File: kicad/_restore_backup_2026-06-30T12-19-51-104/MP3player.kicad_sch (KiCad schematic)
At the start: 0 parts

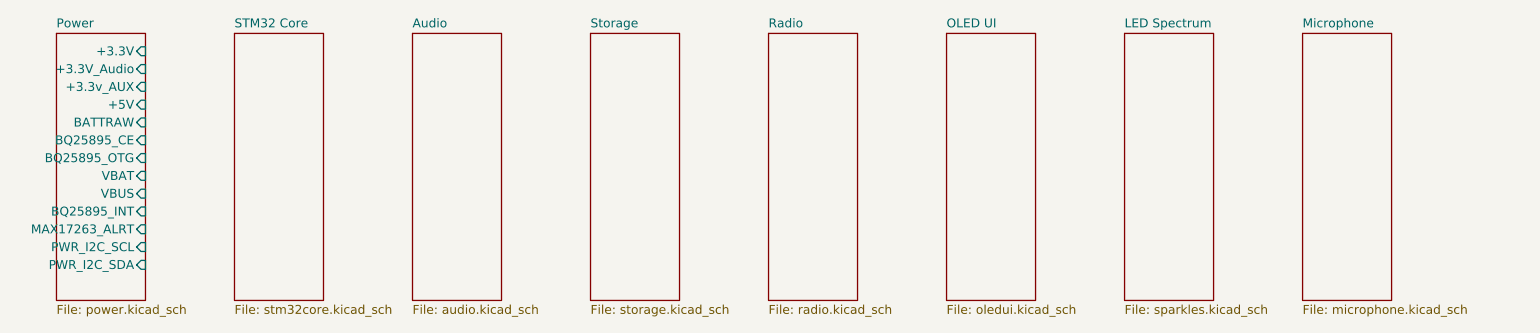
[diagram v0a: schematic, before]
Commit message: updates
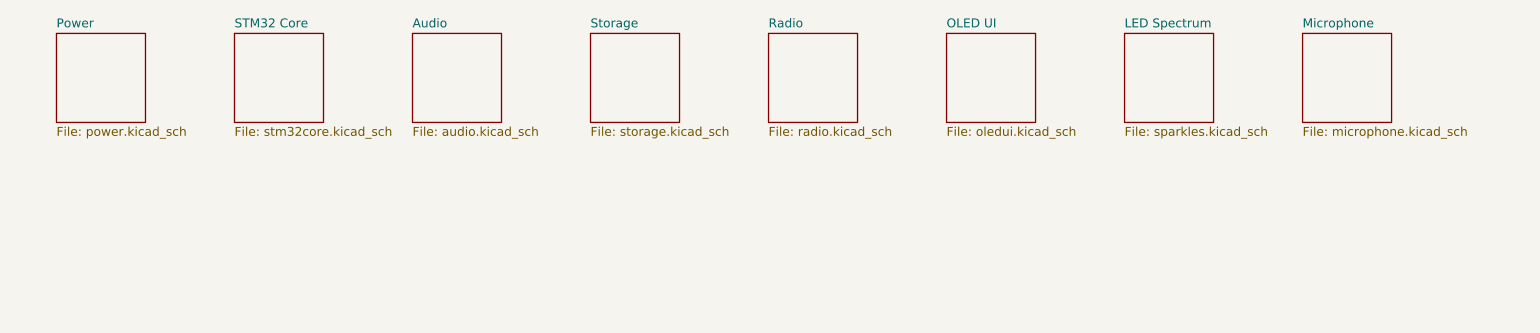
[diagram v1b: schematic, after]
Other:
- sheet Power ports: added none; removed +3.3V, +3.3V_Audio, +3.3v_AUX, +5V, BATTRAW, BQ25895_CE, BQ25895_INT, BQ25895_OTG, MAX17263_ALRT, PWR_I2C_SCL, PWR_I2C_SDA, VBAT, VBUS
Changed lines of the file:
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@@
 	(sheet
 		(at 203.2 25.4)
-		(size 12.7 38.1)
+		(size 12.7 12.7)
 		(exclude_from_sim no)
 		(in_bom yes)
@@
 		)
 		(property "Sheetfile" "microphone.kicad_sch"
-			(at 203.2 64.0846 0)
+			(at 203.2 38.6846 0)
 			(show_name no)
 			(do_not_autoplace no)
@@
 	(sheet
 		(at 25.4 25.4)
-		(size 12.7 38.1)
+		(size 12.7 12.7)
 		(exclude_from_sim no)
 		(in_bom yes)
@@
 		)
 		(property "Sheetfile" "power.kicad_sch"
-			(at 25.4 64.0846 0)
-			(show_name no)
-			(do_not_autoplace no)
-			(effects
-				(font
-					(size 1.27 1.27)
-				)
-				(justify left top)
-			)
-		)
-		(pin "+3.3V" input
-			(at 38.1 27.94 0)
-			(effects
-				(font
-					(size 1.27 1.27)
-				)
-				(justify right)
-			)
-		)
-		(pin "+3.3V_Audio" input
-			(at 38.1 30.48 0)
-			(effects
-				(font
-					(size 1.27 1.27)
-				)
-				(justify right)
-			)
-		)
-		(pin "+5V" input
-			(at 38.1 35.56 0)
-			(effects
-				(font
-					(size 1.27 1.27)
-				)
-				(justify right)
-			)
-		)
-		(pin "BATTRAW" input
-			(at 38.1 38.1 0)
-			(effects
-				(font
-					(size 1.27 1.27)
-				)
-				(justify right)
-			)
-		)
-		(pin "VBAT" input
-			(at 38.1 45.72 0)
-			(effects
-				(font
-					(size 1.27 1.27)
-				)
-				(justify right)
-			)
-		)
-		(pin "VBUS" input
-			(at 38.1 48.26 0)
-			(effects
-				(font
-					(size 1.27 1.27)
-				)
-				(justify right)
-			)
-		)
-		(pin "BQ25895_INT" input
-			(at 38.1 50.8 0)
-			(effects
-				(font
-					(size 1.27 1.27)
-				)
-				(justify right)
-			)
-		)
-		(pin "MAX17263_ALRT" input
-			(at 38.1 53.34 0)
-			(effects
-				(font
-					(size 1.27 1.27)
-				)
-				(justify right)
-			)
-		)
-		(pin "PWR_I2C_SCL" input
-			(at 38.1 55.88 0)
-			(effects
-				(font
-					(size 1.27 1.27)
-				)
-				(justify right)
-			)
-		)
-		(pin "PWR_I2C_SDA" input
-			(at 38.1 58.42 0)
-			(effects
-				(font
-					(size 1.27 1.27)
-				)
-				(justify right)
-			)
-		)
-		(pin "BQ25895_CE" input
-			(at 38.1 40.64 0)
-			(effects
-				(font
-					(size 1.27 1.27)
-				)
-				(justify right)
-			)
-		)
-		(pin "BQ25895_OTG" input
-			(at 38.1 43.18 0)
-			(effects
-				(font
-					(size 1.27 1.27)
-				)
-				(justify right)
-			)
-		)
-		(pin "+3.3v_AUX" input
-			(at 38.1 33.02 0)
-			(effects
-				(font
-					(size 1.27 1.27)
-				)
-				(justify right)
+			(at 25.4 38.6846 0)
+			(show_name no)
+			(do_not_autoplace no)
+			(effects
+				(font
+					(size 1.27 1.27)
+				)
+				(justify left top)
 			)
 		)
@@
 	(sheet
 		(at 152.4 25.4)
-		(size 12.7 38.1)
+		(size 12.7 12.7)
 		(exclude_from_sim no)
 		(in_bom yes)
@@
 		)
 		(property "Sheetfile" "oledui.kicad_sch"
-			(at 152.4 64.0846 0)
+			(at 152.4 38.6846 0)
 			(show_name no)
 			(do_not_autoplace no)
@@
 	(sheet
 		(at 127 25.4)
-		(size 12.7 38.1)
+		(size 12.7 12.7)
 		(exclude_from_sim no)
 		(in_bom yes)
@@
 		)
 		(property "Sheetfile" "radio.kicad_sch"
-			(at 127 64.0846 0)
+			(at 127 38.6846 0)
 			(show_name no)
 			(do_not_autoplace no)
@@
 	(sheet
 		(at 50.8 25.4)
-		(size 12.7 38.1)
+		(size 12.7 12.7)
 		(exclude_from_sim no)
 		(in_bom yes)
@@
 		)
 		(property "Sheetfile" "stm32core.kicad_sch"
-			(at 50.8 64.0846 0)
+			(at 50.8 38.6846 0)
 			(show_name no)
 			(do_not_autoplace no)
@@
 	(sheet
 		(at 177.8 25.4)
-		(size 12.7 38.1)
+		(size 12.7 12.7)
 		(exclude_from_sim no)
 		(in_bom yes)
@@
 		)
 		(property "Sheetfile" "sparkles.kicad_sch"
-			(at 177.8 64.0846 0)
+			(at 177.8 38.6846 0)
 			(show_name no)
 			(do_not_autoplace no)
@@
 	(sheet
 		(at 101.6 25.4)
-		(size 12.7 38.1)
+		(size 12.7 12.7)
 		(exclude_from_sim no)
 		(in_bom yes)
@@
 		)
 		(property "Sheetfile" "storage.kicad_sch"
-			(at 101.6 64.0846 0)
+			(at 101.6 38.6846 0)
 			(show_name no)
 			(do_not_autoplace no)
@@
 	(sheet
 		(at 76.2 25.4)
-		(size 12.7 38.1)
+		(size 12.7 12.7)
 		(exclude_from_sim no)
 		(in_bom yes)
@@
 		)
 		(property "Sheetfile" "audio.kicad_sch"
-			(at 76.2 64.0846 0)
-			(show_name no)
-			(do_not_autoplace no)
+			(at 76.2 38.6846 0)
+			(show_name no)
+			(do_not_autoplace no)
